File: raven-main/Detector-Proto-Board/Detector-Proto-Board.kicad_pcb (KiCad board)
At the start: 2 copper layers, 40.2 x 40.4 mm, 42 parts, among them IC1 ADA4817-1ARDZ-R7, J3 Conn_01x02_Pin, J4 Conn_01x03_Pin, U9 TLV3201AIDCKT

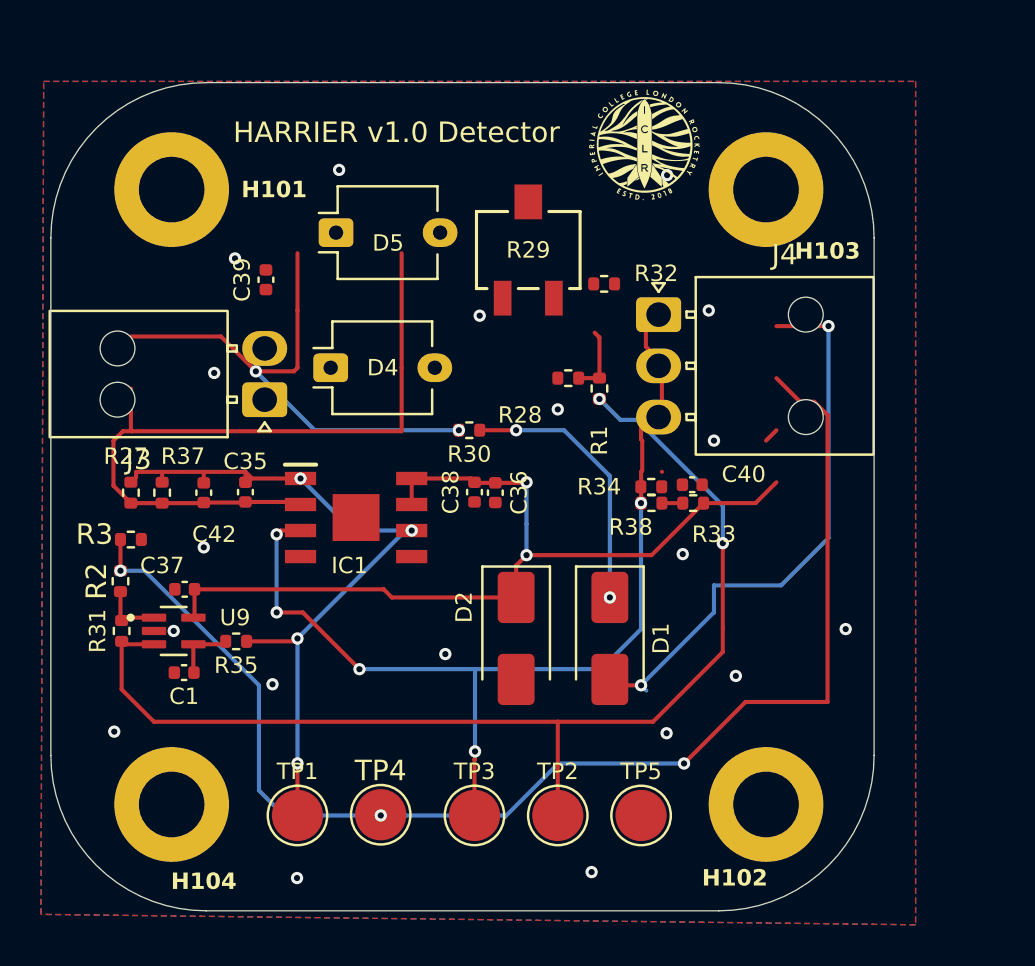
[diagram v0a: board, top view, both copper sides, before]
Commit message: updated detector - need to order
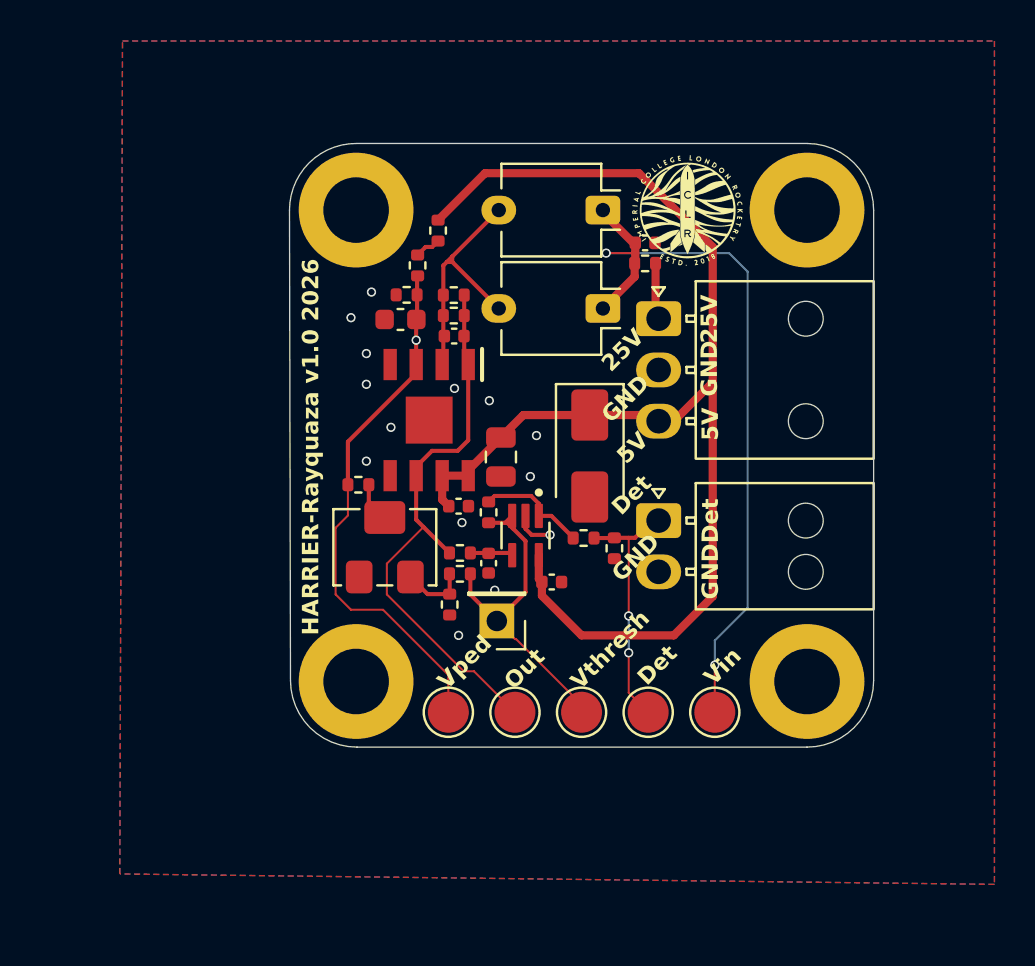
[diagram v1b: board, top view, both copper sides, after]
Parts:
- removed C35, C42: 0.5pF, Capacitor_SMD:C_0402_1005Metric
- removed C36: 10uF, Capacitor_SMD:C_0402_1005Metric
- removed C37, C38, C39: 100nF, Capacitor_SMD:C_0402_1005Metric
- removed C40: 1uF, Capacitor_SMD:C_0402_1005Metric
- removed the D1 at (119.4, 88.9)
- removed the G*** at (105.0, 85.0)
- removed the G*** at (119.0, 84.0)
- removed R27, R37: 1G, Resistor_SMD:R_0402_1005Metric
- removed R29: R_Variable, 3224X:SOT_502E
- removed R30: 10K, Resistor_SMD:R_0402_1005Metric
- removed R31: 390K, Resistor_SMD:R_0402_1005Metric
- removed R32: 33, Resistor_SMD:R_0402_1005Metric
- removed R33, R34: 10k, Resistor_SMD:R_0402_1005Metric
- removed R35: 1.6k, Resistor_SMD:R_0402_1005Metric
- removed R38: 0, Resistor_SMD:R_0402_1005Metric
- removed the TP1 at (104.1, 97.5)
- removed TP4: Detector_Out, TestPoint:TestPoint_Pad_D2.5mm
- added C2: 1uF, Capacitor_SMD:C_0603_1608Metric, F.Cu at (109.2, 73.3)
- added C3: 1pF, Capacitor_SMD:C_0402_1005Metric, F.Cu at (111.8, 74.1)
- added C4: 100nF, Capacitor_SMD:C_0402_1005Metric, F.Cu at (112.0, 82.4)
- added C5: 10uF, Capacitor_SMD:C_0805_2012Metric, F.Cu at (114.1, 80.0)
- added C6: 330pF, Capacitor_SMD:C_0402_1005Metric, F.Cu at (113.5, 85.2)
- added C7: 100nF, Capacitor_SMD:C_0402_1005Metric, F.Cu at (116.5, 86.1)
- added G***: LOGO, LOGO, B.Cu at (117.5, 84.2)
- added J2: Conn_01x01, Connector_PinHeader_2.54mm:PinHeader_1x01_P2.54mm_Vertical, F.Cu at (113.9, 88.0)
- added R10: 0Ω, Resistor_SMD:R_0402_1005Metric, F.Cu at (112.1, 85.7)
- added R11: 1.6kΩ, Resistor_SMD:R_0402_1005Metric, F.Cu at (112.1, 84.7)
- added R12: 390kΩ, Resistor_SMD:R_0402_1005Metric, F.Cu at (113.5, 82.7)
- added R13: 1kΩ, Resistor_SMD:R_0402_1005Metric, F.Cu at (118.1, 84.0)
- added R14: 2kΩ, Resistor_SMD:R_0402_1005Metric, F.Cu at (119.6, 84.5)
- added R4: 10kΩ, Resistor_SMD:R_0402_1005Metric, F.Cu at (109.5, 72.1)
- added R5: 1GΩ, Resistor_SMD:R_0402_1005Metric, F.Cu at (111.8, 73.1)
- added R6: 1GΩ, Resistor_SMD:R_0402_1005Metric, F.Cu at (111.8, 72.1)
- added R7: 33Ω, Resistor_SMD:R_0402_1005Metric, F.Cu at (107.1, 81.4)
- added RV1: 3214W-1-102E, Potentiometer_SMD:Potentiometer_Bourns_3214W_Vertical, F.Cu at (108.4, 84.5)
- added TP2: 25V, TestPoint:TestPoint_Pad_D2.0mm, F.Cu at (124.5, 92.5)
- added TP6: Detector_Out, TestPoint:TestPoint_Pad_D2.0mm, F.Cu at (121.2, 92.5)
- C1: value 330p -> 100nF 50V
- R1: value 0 -> 10kΩ
- R2: value 1k -> 10kΩ
- R3: value 2k -> 0Ω
- R9: renamed from R28; value 100k -> 100kΩ
- TP1: renamed from TP3; footprint TestPoint:TestPoint_Pad_D2.5mm -> TestPoint:TestPoint_Pad_D2.0mm
- TP3: renamed from TP2; footprint TestPoint:TestPoint_Pad_D2.5mm -> TestPoint:TestPoint_Pad_D2.0mm
- TP5: value GND -> OUT; footprint TestPoint:TestPoint_Pad_D2.5mm -> TestPoint:TestPoint_Pad_D2.0mm
- moved C1 30.7 mm to (121.1, 69.6), turned to 0 degrees
- moved R2 23.1 mm to (111.0, 69.0), turned to -90 degrees
- moved J3 20.1 mm to (121.8, 83.2), turned to 0 degrees
- moved R3 19.4 mm to (110.0, 70.7), turned to -90 degrees
- moved U1 17.8 mm to (115.3, 83.9), turned to -90 degrees
- moved D1 13.6 mm to (119.0, 72.8), turned to 180 degrees
- moved D2 13.1 mm to (119.0, 68.0), turned to 180 degrees
- moved R9 12.5 mm to (111.6, 87.2), turned to -90 degrees
- moved H4 10.8 mm to (107.0, 91.0)
- moved D3 9.60 mm to (118.4, 80.0)
- moved H1 9.06 mm to (107.0, 68.0)
- moved TP5 7.95 mm to (114.8, 92.5), turned to 90 degrees
- moved R1 6.50 mm to (121.1, 70.6), turned to 180 degrees
- moved H2 6.32 mm to (129.0, 91.0)
- moved IC1 5.94 mm to (110.6, 78.2), turned to -90 degrees
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- renumbered D4 to D1, D5 to D2, D2 to D3, H101 to H1, H102 to H2, H103 to H3, H104 to H4, J4 to J1, U9 to U1
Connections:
- C1 pad 1: Net-(U9-IN-) -> Net-(D1-K)
- D1 pad 1: Net-(D4-K) -> Net-(D1-K)
- D2 pad 1: Net-(D4-K) -> Net-(D1-K)
- J1 pad 1: Net-(D1-A2) -> +25V
- R1 pad 1: Net-(R1-Pad1) -> +25V
- R1 pad 2: /V_thresh -> Net-(D1-K)
- R2 pad 1: Net-(U9-OUT) -> +5V
- R2 pad 2: /Detector_Out -> Net-(R2-Pad2)
- R3 pad 1: /Detector_Out -> Net-(R2-Pad2)
- R3 pad 2: GND -> /Vped
- R9 pad 1: Net-(R1-Pad1) -> Net-(R10-Pad1)
- TP5 pad 1: GND -> /OUT
- U1 pad 1: Net-(U9-OUT) -> /Detector_Out_5V
- U1 pad 4: Net-(U9-IN-) -> Net-(U1-IN-)
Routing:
- net /Detector_Out: track 63.6 -> 12.4 mm, vias 3 -> 2
- net /V_thresh: track 55.3 -> 17.3 mm, vias 2 -> 0
- net Net-(D1-K): track 0.00 -> 37.0 mm, vias 0 -> 2
- net Net-(D1-A2): track 27.8 -> 0.00 mm, vias 2 -> 0
- net Net-(D4-K): track 25.6 -> 0.00 mm, vias 2 -> 0
- net Net-(D1-A): track 36.8 -> 12.4 mm
- net +5V: track 43.7 -> 62.4 mm, vias 2 -> 0
- net /Vped: track 42.7 -> 26.2 mm, vias 5 -> 1
- net +25V: track 13.2 -> 3.39 mm, vias 2 -> 0
- net /OUT: track 36.3 -> 27.8 mm, vias 4 -> 0
- net /Detector_Out_5V: track 0.00 -> 5.46 mm
- net Net-(R29-Pad2): track 4.07 -> 0.00 mm
- net Net-(R1-Pad1): track 3.33 -> 0.00 mm
- net Net-(R10-Pad1): track 0.00 -> 3.26 mm
- net Net-(U9-OUT): track 3.07 -> 0.00 mm
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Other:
- board size 40.2 x 40.4 mm -> 28.5 x 29.5 mm
- board text added: "25V"
- board text added: "5V"
- board text added: "Det"
- board text added: "GND"
- board text added: "HARRIER-Rayquaza v1.0"
- board text added: "HARRIER-Rayquaza v1.0 2026"
- board text added: "Out"
- board text added: "Vin"
- board text added: "Vped"
- board text added: "Vthresh"
- board text removed: "HARRIER v1.0 Detector"
